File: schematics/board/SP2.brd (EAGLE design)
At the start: 30 x 46 mm, 13 parts

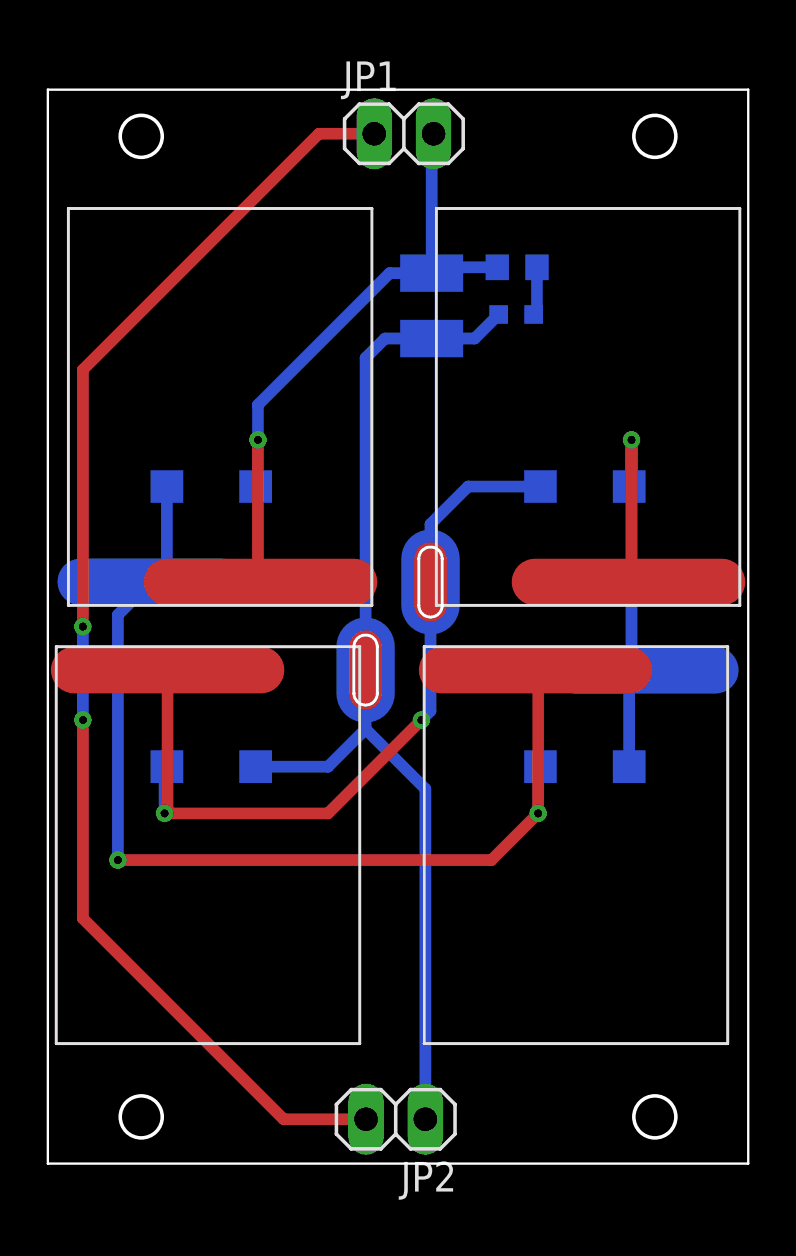
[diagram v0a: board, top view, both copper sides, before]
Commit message: Подготовлены платы SP и mtr
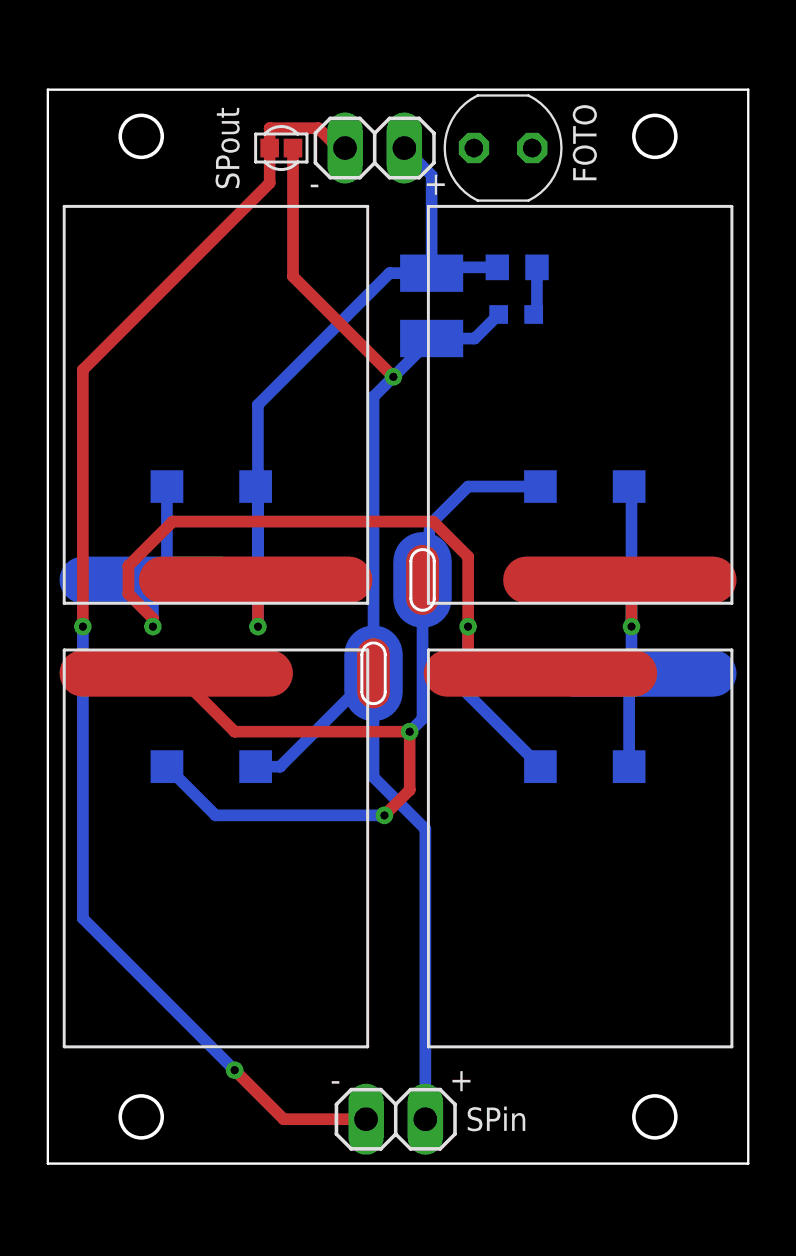
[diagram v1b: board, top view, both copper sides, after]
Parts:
- added FOTO: VT93N1VERT, KNPN-2023:VT93N1-VERT
- added U$7: (no value), KNPN-2023:VIAS-CONNECT
- U$1, U$2: device CanCubeSat:SOLAR_1-2 -> KNPN-2023:SOLAR_1-2
- U$3, U$4: device CanCubeSat:SOLAR_0-2 -> KNPN-2023:SOLAR_0-2
- moved JP1 1.39 mm to (14.0, 43.5)
- moved U$4 0.37 mm to (7.20, 13.5)
- moved U$3 0.35 mm to (22.8, 32.5)
- moved U$2 0.23 mm to (22.8, 13.5)
- moved U$1 0.20 mm to (7.20, 32.5)
- renumbered JP2 to SP-OUT, LED1 to PWR
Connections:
- net SP+-: now also U$7.1
- net SP-: now also U$7.2
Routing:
- net SP+-: track 45.5 -> 57.0 mm, vias 0 -> 1
- net SP+: track 28.8 -> 36.6 mm
- net N$2: track 22.7 -> 15.0 mm
- net N$3: track 34.8 -> 39.9 mm
- net N$1: track 43.9 -> 40.7 mm
- net SP-: track 55.9 -> 56.4 mm
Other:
- board text added: "+"
- board text added: "-"
- board text added: "SPin"
- board text added: "SPout"
